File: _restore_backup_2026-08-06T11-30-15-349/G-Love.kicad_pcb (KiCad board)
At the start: 2 copper layers, 218.5 x 139 mm, 151 parts, among them J4 XLR5_Ground, U1 ATMEGA2561-16AU, U10 74HC4052, U11 74HC4052, U14 TPS2113APWR, U17 6N137, U18 MAX485E, U2 ATMega328P, U3 TXS0108EPWR, U4 ICM-42688-P_I2C, U5 TXS0104E, U6 Hall Sensor A3144, U9 TUSB321, Y1 16MHz, Y2 16MHz

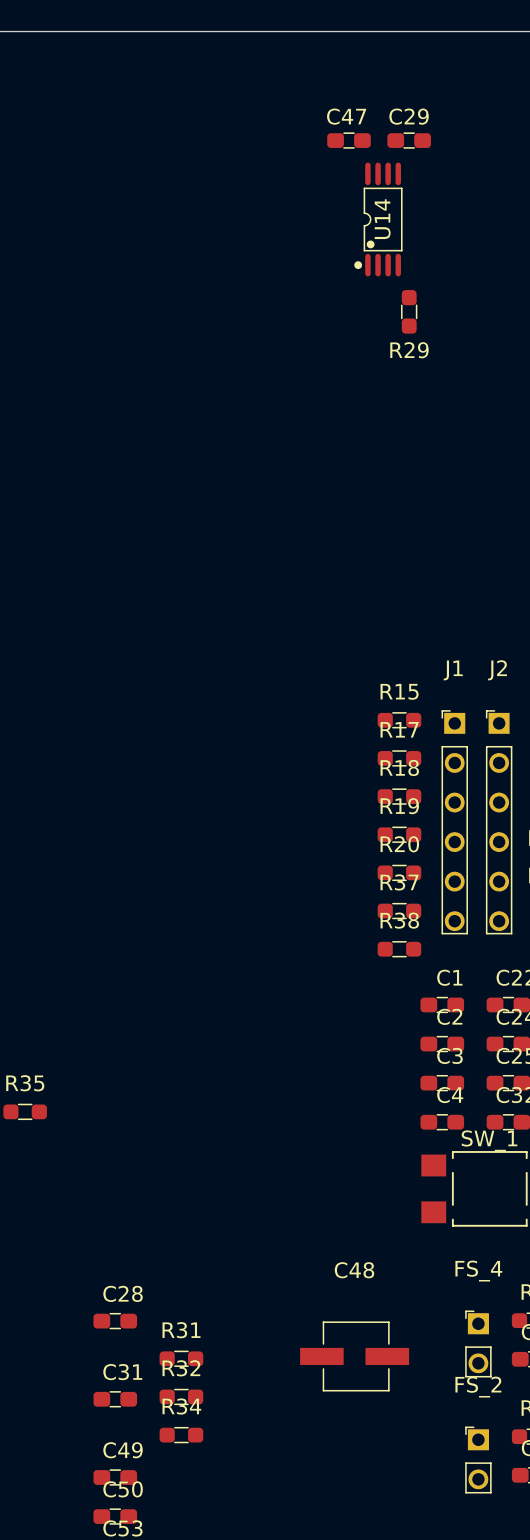
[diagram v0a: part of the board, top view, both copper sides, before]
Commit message: osekour
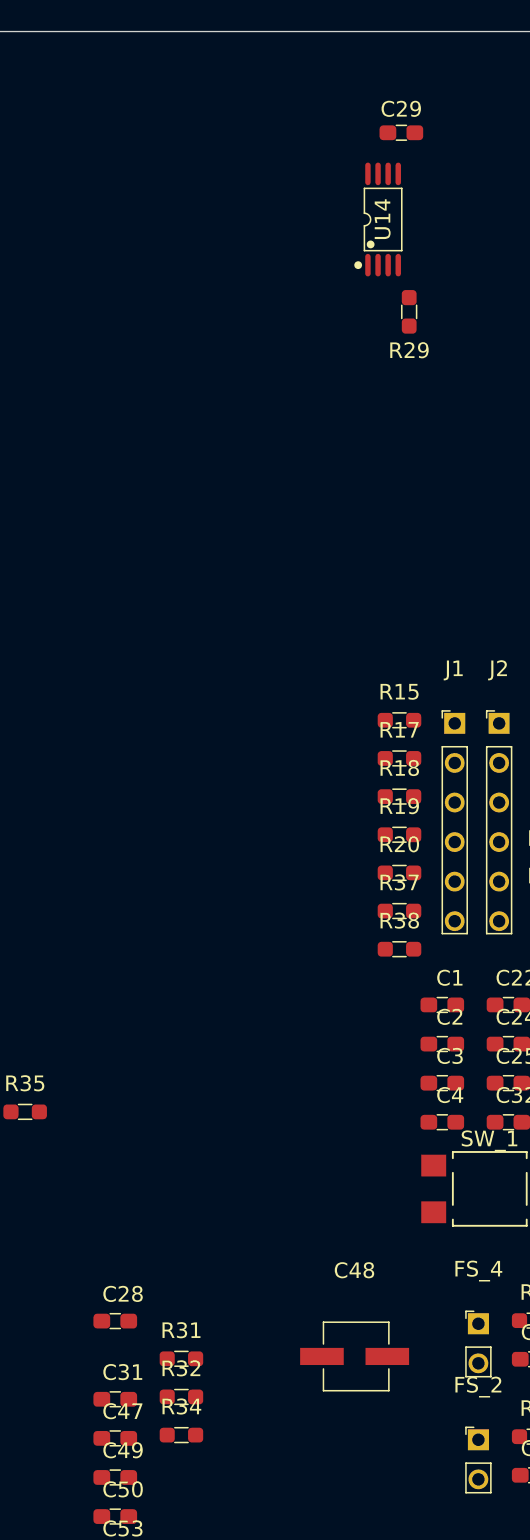
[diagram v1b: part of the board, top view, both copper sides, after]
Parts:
- moved C47 84.7 mm to (110.1, 115.8), turned to 0 degrees
- moved C29 0.71 mm to (128.5, 32.0)
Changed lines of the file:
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@@
 	(footprint "MyGlove:Capacitor_0603"
 		(layer "F.Cu")
-		(at 129 32.5 180)
+		(at 128.5 32 180)
 		(property "Reference" "C29"
 			(at 0 1.5 0)
@@
 	(footprint "MyGlove:Capacitor_0603"
 		(layer "F.Cu")
-		(at 125.1375 32.5 180)
+		(at 110.125 115.835)
 		(property "Reference" "C47"
-			(at 0.1375 1.5 0)
+			(at 0.51 -1.71 0)
 			(unlocked yes)
 			(layer "F.SilkS")
@@
 		)
 		(property "Value" "1uF"
-			(at 0 1.2 180)
+			(at 0 1.2 0)
 			(unlocked yes)
 			(layer "F.Fab")
@@
 		)
 		(property "Datasheet" ""
-			(at 0 0 180)
+			(at 0 0 0)
 			(unlocked yes)
 			(layer "F.Fab")
@@
 		)
 		(property "Description" "Capacitor"
-			(at 0 0 180)
+			(at 0 0 0)
 			(unlocked yes)
 			(layer "F.Fab")
@@
 		)
 		(property "Minimum quantity per command" ""
-			(at 0 0 180)
+			(at 0 0 0)
 			(unlocked yes)
 			(layer "F.Fab")
@@
 		)
 		(property "Price" "4.39/50"
-			(at 0 0 180)
+			(at 0 0 0)
 			(unlocked yes)
 			(layer "F.Fab")
@@
 		)
 		(property "SUPPLIER" "https://www.lcsc.com/product-detail/C15849.html"
-			(at 0 0 180)
+			(at 0 0 0)
 			(unlocked yes)
 			(layer "F.Fab")
@@
 		(duplicate_pad_numbers_are_jumpers no)
 		(fp_line
+			(start -0.325 -0.475)
+			(end 0.3275 -0.475)
+			(stroke
+				(width 0.1)
+				(type default)
+			)
+			(layer "F.SilkS")
+		)
+		(fp_line
 			(start 0.3275 0.475)
 			(end -0.325 0.475)
@@
 		)
 		(fp_line
-			(start -0.325 -0.475)
-			(end 0.3275 -0.475)
-			(stroke
-				(width 0.1)
-				(type default)
-			)
-			(layer "F.SilkS")
+			(start -1.6 -0.73)
+			(end -1.6 0.73)
+			(stroke
+				(width 0.05)
+				(type default)
+			)
+			(layer "F.CrtYd")
+		)
+		(fp_line
+			(start -1.6 0.73)
+			(end 1.6 0.73)
+			(stroke
+				(width 0.05)
+				(type default)
+			)
+			(layer "F.CrtYd")
+		)
+		(fp_line
+			(start 1.6 -0.73)
+			(end -1.6 -0.73)
+			(stroke
+				(width 0.05)
+				(type default)
+			)
+			(layer "F.CrtYd")
 		)
 		(fp_line
@@
 			(layer "F.CrtYd")
 		)
-		(fp_line
-			(start 1.6 -0.73)
-			(end -1.6 -0.73)
-			(stroke
-				(width 0.05)
-				(type default)
-			)
-			(layer "F.CrtYd")
-		)
-		(fp_line
-			(start -1.6 0.73)
-			(end 1.6 0.73)
-			(stroke
-				(width 0.05)
-				(type default)
-			)
-			(layer "F.CrtYd")
-		)
-		(fp_line
-			(start -1.6 -0.73)
-			(end -1.6 0.73)
-			(stroke
-				(width 0.05)
-				(type default)
-			)
-			(layer "F.CrtYd")
-		)
 		(fp_text user "${REFERENCE}"
-			(at 0 2.5 180)
+			(at 0 2.5 0)
 			(unlocked yes)
 			(layer "F.Fab")
@@
 		)
 		(pad "1" smd roundrect
-			(at -0.8625 0 180)
+			(at -0.8625 0)
 			(size 1.075 0.95)
 			(layers "F.Cu" "F.Mask" "F.Paste")
@@
 		)
 		(pad "2" smd roundrect
-			(at 0.865 0 180)
+			(at 0.865 0)
 			(size 1.075 0.95)
 			(layers "F.Cu" "F.Mask" "F.Paste")
